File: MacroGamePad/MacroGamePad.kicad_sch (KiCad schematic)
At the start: 14 parts, among them SW1 SW_Push, SW2 SW_Push, SW3 SW_Push, SW4 SW_Push, SW5 SW_Push, SW6 RotaryEncoder_Switch, U1 MOUDLE-SEEEDUINO-XIAO

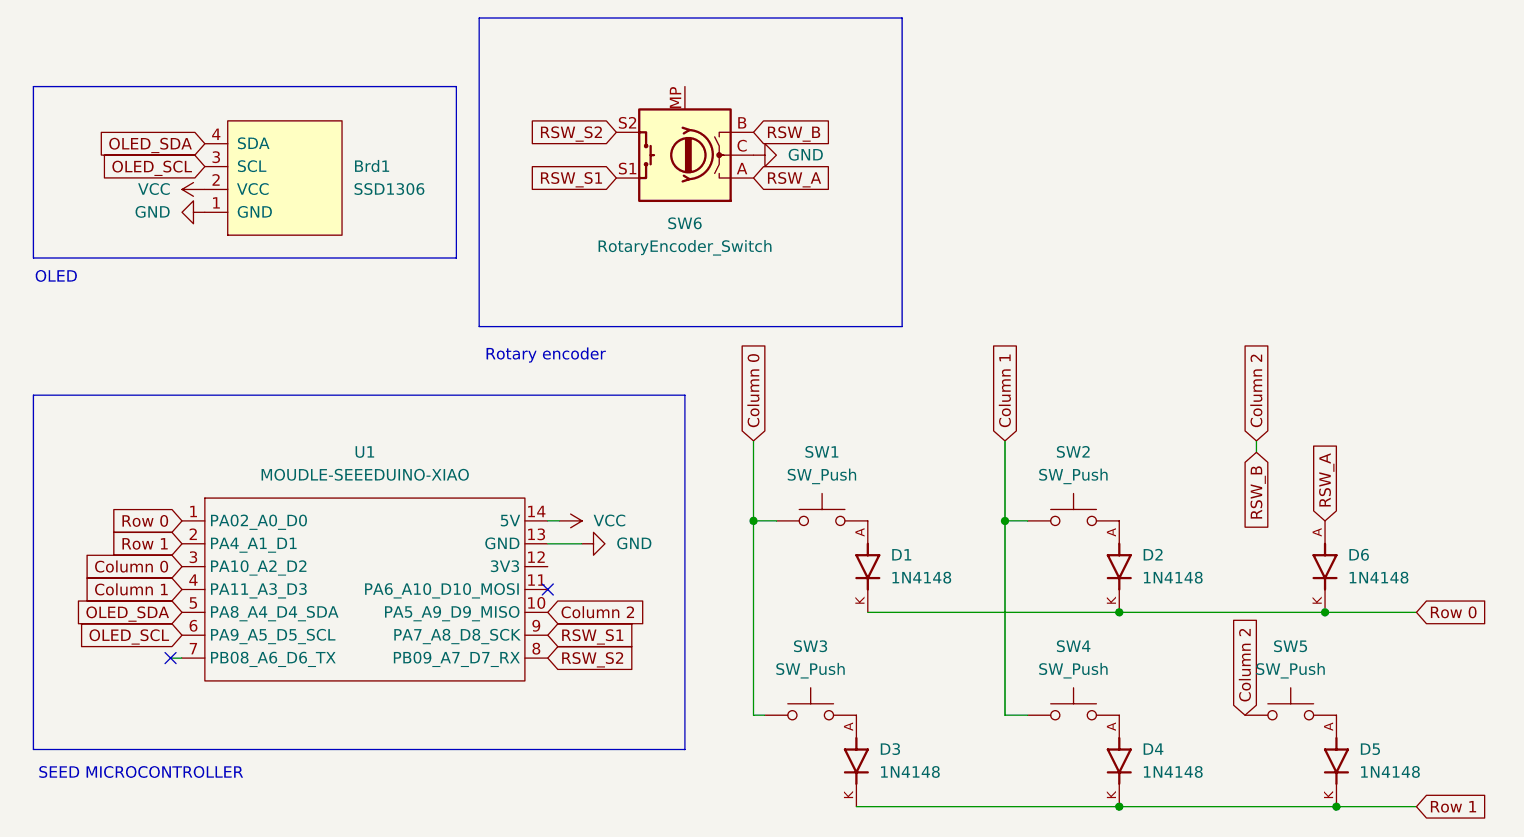
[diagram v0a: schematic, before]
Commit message: PCB finished
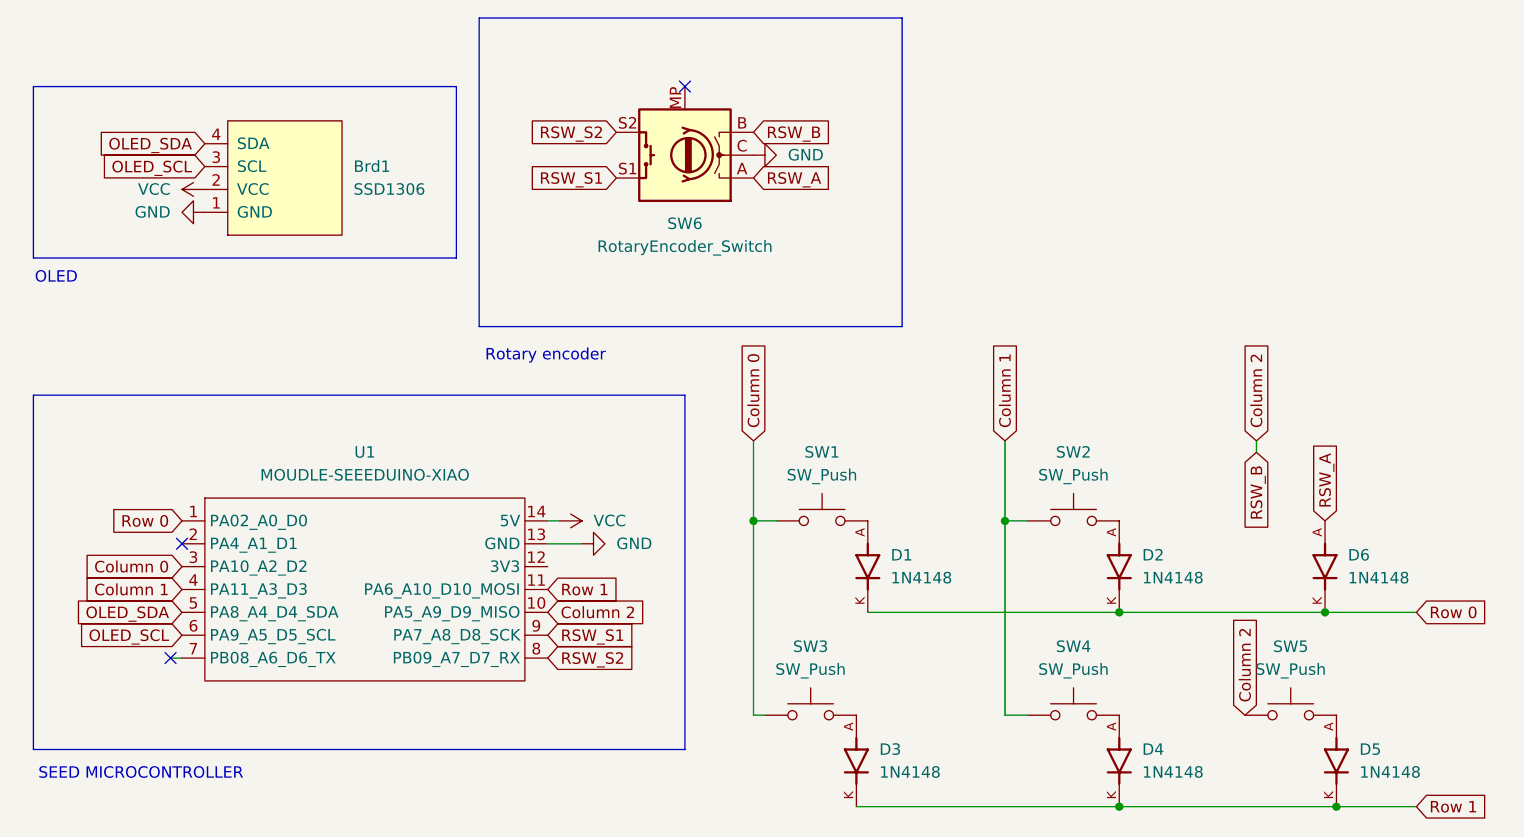
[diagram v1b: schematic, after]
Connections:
- net Row 1: now also U1.11 (PA6_A10_D10_MOSI); no longer U1.2 (PA4_A1_D1)
- no-connect marks 2 -> 3
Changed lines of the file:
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@@
+	)
+	(no_connect
+		(at 119.38 22.86)
 	)
 	(no_connect
@@
 	)
 	(no_connect
-		(at 104.14 78.74)
+		(at 63.5 73.66)
 	)
 	(wire
@@
 	(global_label "Row 1"
 		(shape input)
-		(at 63.5 73.66 180)
-		(fields_autoplaced yes)
-		(effects
-			(font
-				(size 1.27 1.27)
-			)
-			(justify right)
-		)
-		(property "Intersheetrefs" "${INTERSHEET_REFS}"
-			(at 54.5882 73.66 0)
-			(effects
-				(font
-					(size 1.27 1.27)
-				)
-				(justify right)
-				(hide yes)
-			)
+		(at 104.14 78.74 0)
+		(fields_autoplaced yes)
+		(effects
+			(font
+				(size 1.27 1.27)
+			)
+			(justify left)
+		)
+		(property "Intersheetrefs" "${INTERSHEET_REFS}"
+			(at 113.0518 78.74 0)
+			(effects
+				(font
+					(size 1.27 1.27)
+				)
+				(justify left)
+				(hide yes)
+			)
